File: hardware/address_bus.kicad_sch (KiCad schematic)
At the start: 17 parts, among them Q7 BC557, Q8 BC557, U2 74LS06N, U5 74HC595, U6 74HC595, U7 74HC595

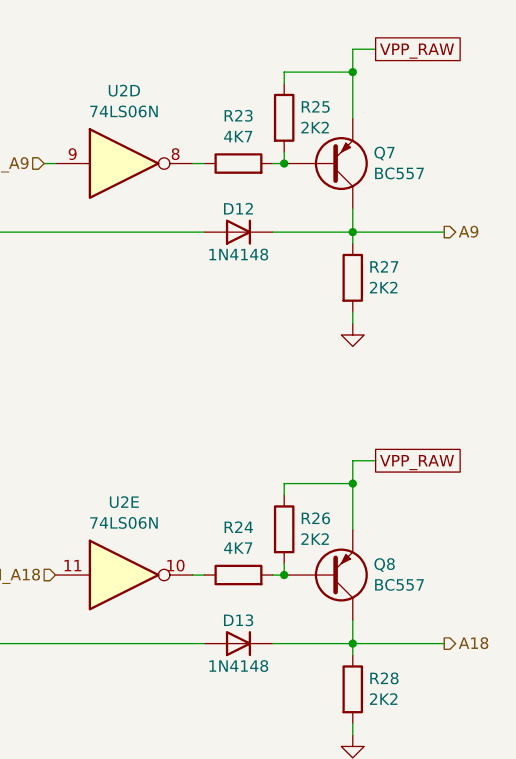
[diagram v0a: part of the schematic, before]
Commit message: Rev.E. Updated specifications document and hardware design.
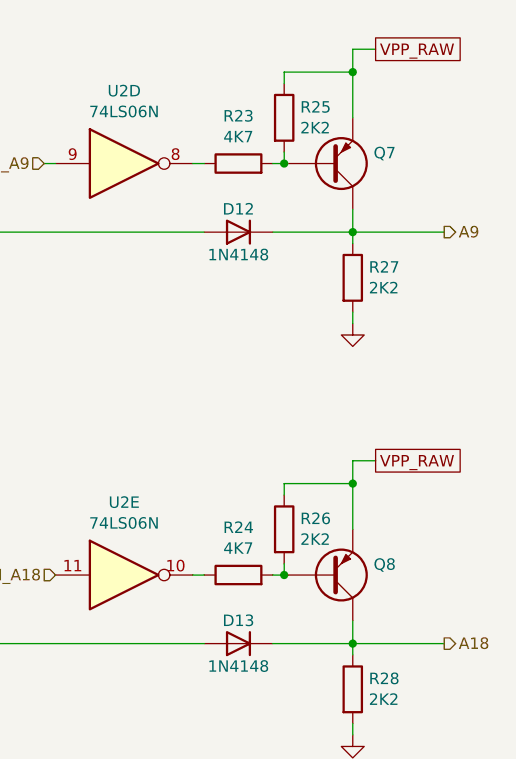
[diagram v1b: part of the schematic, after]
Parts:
- Q7, Q8: value BC557 -> (none); footprint Package_TO_SOT_THT:TO-92_Inline_Wide -> (none)
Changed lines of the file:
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@@
       (effects (font (size 1.27 1.27)) (justify left))
     )
-    (property "Value" "BC557" (id 1) (at 185.1914 77.343 0)
+    (property "Value" "" (id 1) (at 185.1914 77.343 0)
       (effects (font (size 1.27 1.27)) (justify left))
     )
-    (property "Footprint" "Package_TO_SOT_THT:TO-92_Inline_Wide" (id 2) (at 185.42 74.295 0)
+    (property "Footprint" "" (id 2) (at 185.42 74.295 0)
       (effects (font (size 1.27 1.27) italic) (justify left) hide)
     )
@@
       (effects (font (size 1.27 1.27)) (justify left))
     )
-    (property "Value" "BC557" (id 1) (at 185.1914 123.063 0)
+    (property "Value" "" (id 1) (at 185.1914 123.063 0)
       (effects (font (size 1.27 1.27)) (justify left))
     )
-    (property "Footprint" "Package_TO_SOT_THT:TO-92_Inline_Wide" (id 2) (at 185.42 120.015 0)
+    (property "Footprint" "" (id 2) (at 185.42 120.015 0)
       (effects (font (size 1.27 1.27) italic) (justify left) hide)
     )
